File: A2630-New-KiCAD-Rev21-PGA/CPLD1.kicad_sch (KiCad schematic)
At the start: 18 parts, among them CN600 CPLD0, CN601 CPLD1, CN602 CPLD2, J600 IDE DISABLE, U600 XC9572XL-VQ64, U601 XC95144XL-TQ144, U602 XC95144XL-TQ144

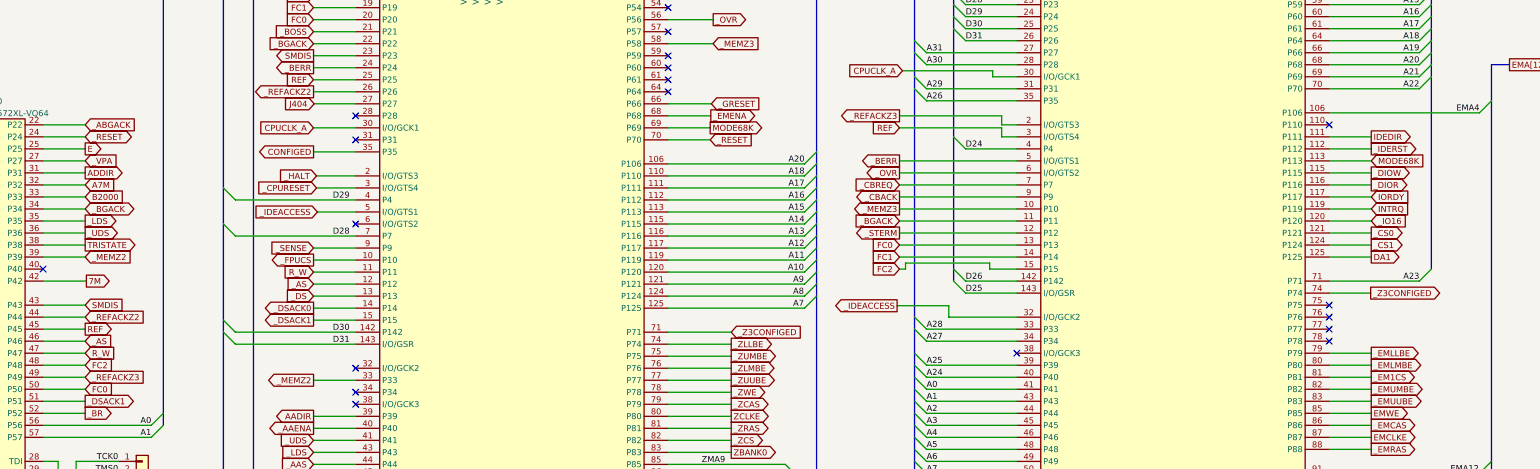
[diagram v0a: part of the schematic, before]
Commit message: Add files via upload
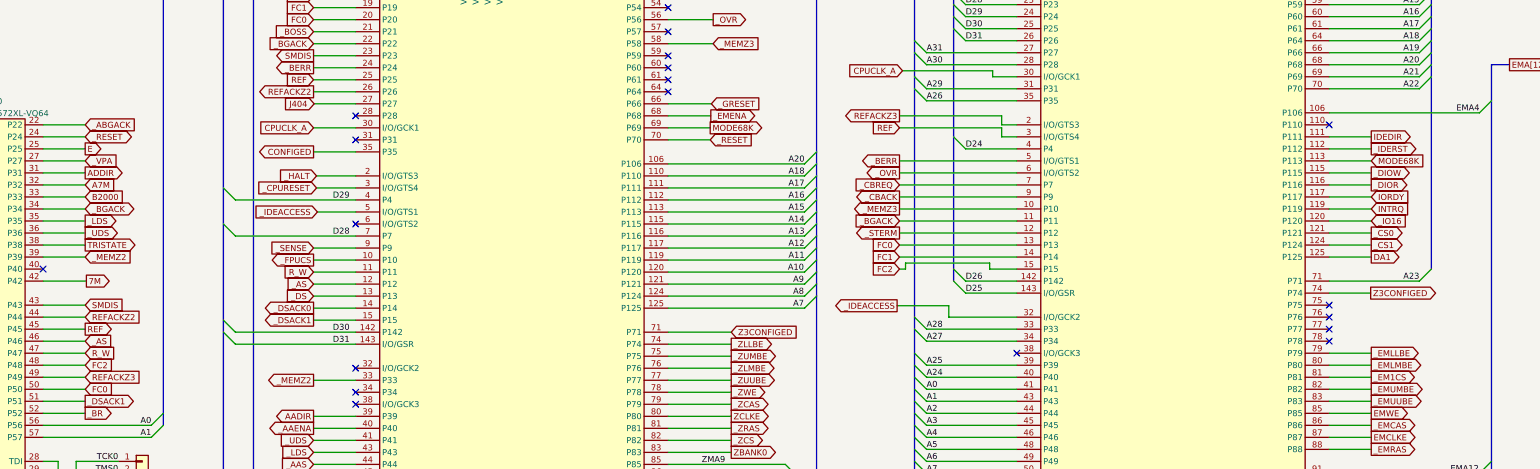
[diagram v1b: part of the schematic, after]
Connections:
- net _REFACKZ2 renamed REFACKZ2
- net _REFACKZ3 renamed REFACKZ3
- net _Z3CONFIGED renamed Z3CONFIGED
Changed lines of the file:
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@@
     )
   )
-  (global_label "_REFACKZ3" (shape output) (at 275.59 92.71 180) (fields_autoplaced)
-    (effects (font (size 1.27 1.27)) (justify right))
-    (property "Intersheet References" "${INTERSHEET_REFS}" (id 0) (at 262.7429 92.6306 0)
+  (global_label "REFACKZ3" (shape output) (at 275.59 92.71 180) (fields_autoplaced)
+    (effects (font (size 1.27 1.27)) (justify right))
+    (property "Intersheet References" "${INTERSHEET_REFS}" (id 0) (at 263.7106 92.6306 0)
       (effects (font (size 1.27 1.27)) (justify right) hide)
     )
@@
     )
   )
-  (global_label "_REFACKZ2" (shape input) (at 103.505 135.255 0) (fields_autoplaced)
-    (effects (font (size 1.27 1.27)) (justify left))
-    (property "Intersheet References" "${INTERSHEET_REFS}" (id 0) (at 116.3521 135.1756 0)
+  (global_label "REFACKZ2" (shape input) (at 103.505 135.255 0) (fields_autoplaced)
+    (effects (font (size 1.27 1.27)) (justify left))
+    (property "Intersheet References" "${INTERSHEET_REFS}" (id 0) (at 115.3844 135.1756 0)
       (effects (font (size 1.27 1.27)) (justify left) hide)
     )
@@
     )
   )
-  (global_label "_REFACKZ2" (shape output) (at 151.765 87.63 180) (fields_autoplaced)
-    (effects (font (size 1.27 1.27)) (justify right))
-    (property "Intersheet References" "${INTERSHEET_REFS}" (id 0) (at 138.9179 87.5506 0)
+  (global_label "REFACKZ2" (shape output) (at 151.765 87.63 180) (fields_autoplaced)
+    (effects (font (size 1.27 1.27)) (justify right))
+    (property "Intersheet References" "${INTERSHEET_REFS}" (id 0) (at 139.8856 87.5506 0)
       (effects (font (size 1.27 1.27)) (justify right) hide)
     )
@@
     )
   )
-  (global_label "_Z3CONFIGED" (shape input) (at 240.03 138.43 0) (fields_autoplaced)
-    (effects (font (size 1.27 1.27)) (justify left))
-    (property "Intersheet References" "${INTERSHEET_REFS}" (id 0) (at 255.0542 138.3506 0)
+  (global_label "Z3CONFIGED" (shape input) (at 240.03 138.43 0) (fields_autoplaced)
+    (effects (font (size 1.27 1.27)) (justify left))
+    (property "Intersheet References" "${INTERSHEET_REFS}" (id 0) (at 254.0866 138.3506 0)
       (effects (font (size 1.27 1.27)) (justify left) hide)
     )
@@
     )
   )
-  (global_label "_REFACKZ3" (shape input) (at 103.505 147.955 0) (fields_autoplaced)
-    (effects (font (size 1.27 1.27)) (justify left))
-    (property "Intersheet References" "${INTERSHEET_REFS}" (id 0) (at 116.3521 147.8756 0)
+  (global_label "REFACKZ3" (shape input) (at 103.505 147.955 0) (fields_autoplaced)
+    (effects (font (size 1.27 1.27)) (justify left))
+    (property "Intersheet References" "${INTERSHEET_REFS}" (id 0) (at 115.3844 147.8756 0)
       (effects (font (size 1.27 1.27)) (justify left) hide)
     )
@@
     )
   )
-  (global_label "_Z3CONFIGED" (shape output) (at 375.158 130.175 0) (fields_autoplaced)
-    (effects (font (size 1.27 1.27)) (justify left))
-    (property "Intersheet References" "${INTERSHEET_REFS}" (id 0) (at 390.1822 130.0956 0)
-      (effects (font (size 1.27 1.27)) (justify left) hide)
-    )
+  (global_label "Z3CONFIGED" (shape output) (at 375.158 130.175 0) (fields_autoplaced)
+    (effects (font (size 1.27 1.27)) (justify left))
+    (property "Intersheet References" "${INTERSHEET_REFS}" (id 0) (at 389.2146 130.0956 0)
+      (effects (font (size 1.27 1.27)) (justify left) hide)
+    )
